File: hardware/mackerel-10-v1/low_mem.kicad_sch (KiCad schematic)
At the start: 4 parts, among them U2 AS6C4008-55PCN, U3 SST39SF040, U4 AS6C4008-55PCN, U5 SST39SF040

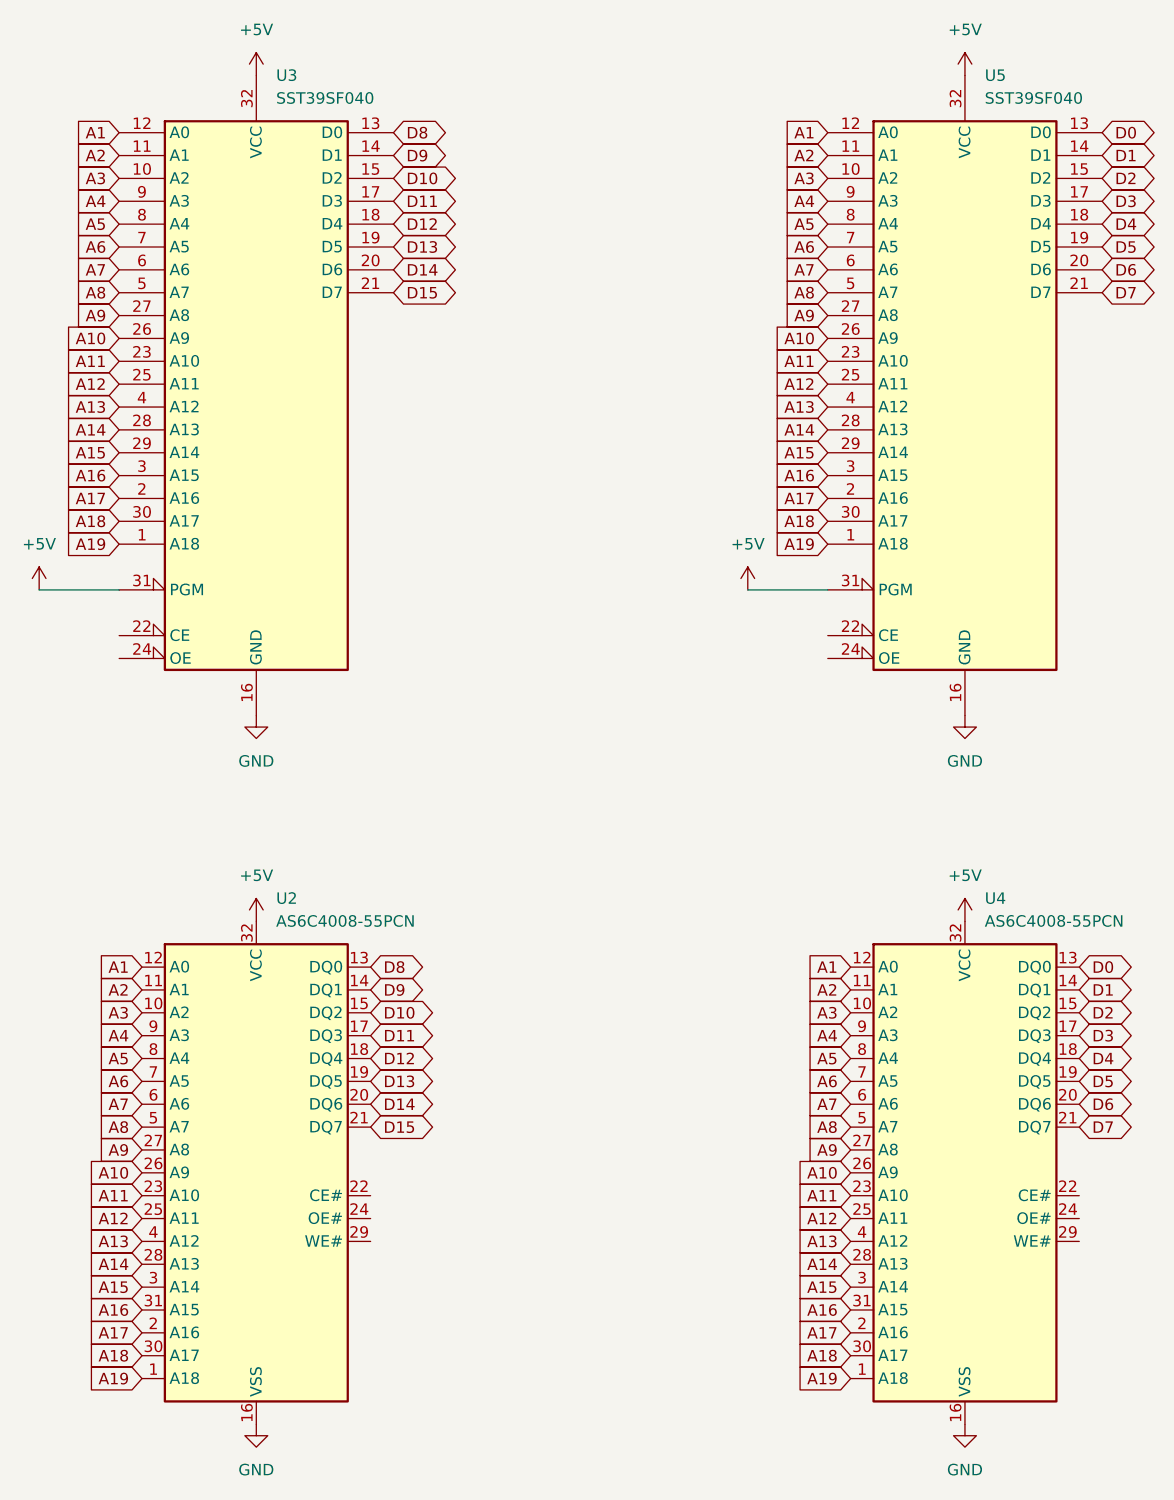
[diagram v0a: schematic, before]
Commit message: Trying to figure out Mackerel-10 components
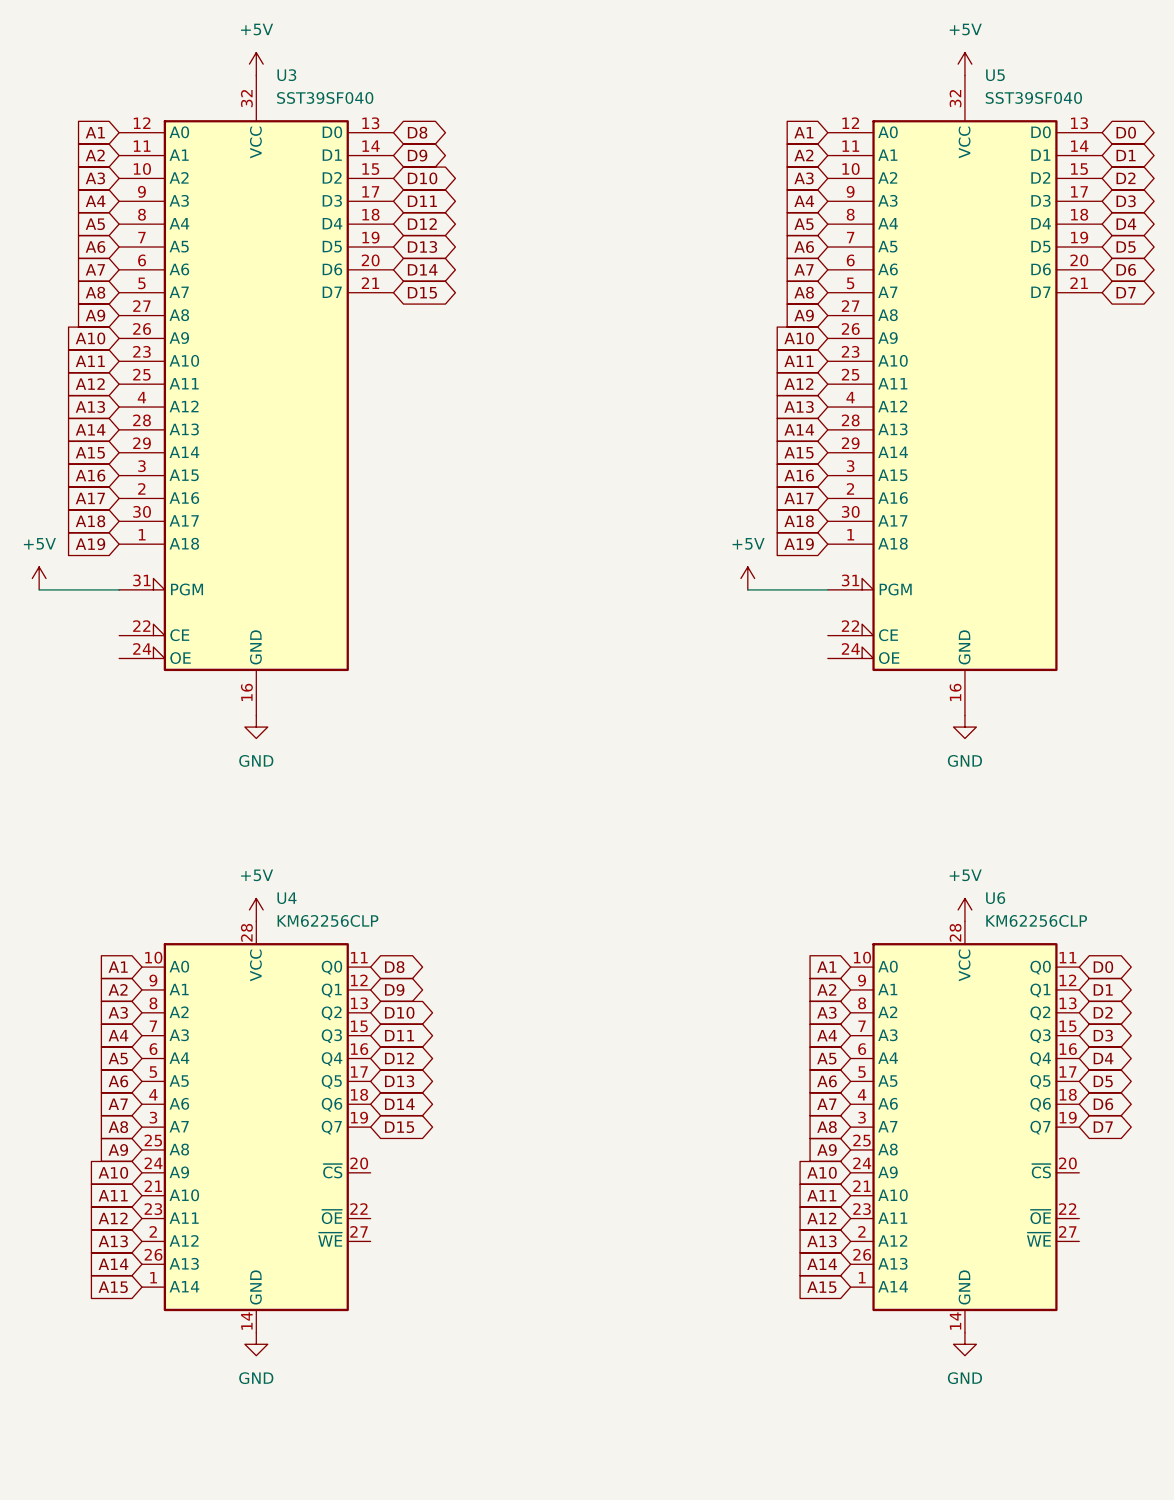
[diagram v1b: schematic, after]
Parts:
- removed U2, U4: AS6C4008-55PCN, Package_DIP:DIP-32_W15.24mm, symbol Memory_RAM:AS6C4008-55PCN
- added U4, U6: KM62256CLP, Package_DIP:DIP-28_W15.24mm, symbol Memory_RAM:KM62256CLP
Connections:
- net +5V: now also U4.28 (VCC), U6.28 (VCC)
- net A1: now also U4.10 (A0), U6.10 (A0)
- net A10: now also U4.24 (A9), U6.24 (A9)
- net A11: now also U4.21 (A10), U6.21 (A10)
- net A12: now also U4.23 (A11), U6.23 (A11)
- net A13: now also U4.2 (A12), U6.2 (A12)
- net A14: now also U4.26 (A13), U6.26 (A13)
- net A15: now also U4.1 (A14), U6.1 (A14)
- net A2: now also U4.9 (A1), U6.9 (A1)
- net A3: now also U4.8 (A2), U6.8 (A2)
- net A4: now also U4.7 (A3), U6.7 (A3)
- net A5: now also U4.6 (A4), U6.6 (A4)
- net A6: now also U4.5 (A5), U6.5 (A5)
- net A7: now also U4.4 (A6), U6.4 (A6)
- net A8: now also U4.3 (A7), U6.3 (A7)
- net A9: now also U4.25 (A8), U6.25 (A8)
- net D0: now also U6.11 (Q0)
- net D1: now also U6.12 (Q1)
- net D10: now also U4.13 (Q2)
- net D11: now also U4.15 (Q3)
- net D12: now also U4.16 (Q4)
- net D13: now also U4.17 (Q5)
- net D14: now also U4.18 (Q6)
- net D15: now also U4.19 (Q7)
- net D2: now also U6.13 (Q2)
- net D3: now also U6.15 (Q3)
- net D4: now also U6.16 (Q4)
- net D5: now also U6.17 (Q5)
- net D6: now also U6.18 (Q6)
- net D7: now also U6.19 (Q7)
- net D8: now also U4.11 (Q0)
- net D9: now also U4.12 (Q1)
- net GND: now also U4.14 (GND), U6.14 (GND)
